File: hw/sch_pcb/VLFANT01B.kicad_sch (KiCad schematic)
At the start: 9 parts, among them J1 RJ45_RJHSE-5384, J2 RJ45_RJHSE-5384, J3 RJ45_RJHSE-5384, J7 SMA, J9 JUMP_3X2, M1 HOLE, M2 HOLE, M3 HOLE, M4 HOLE

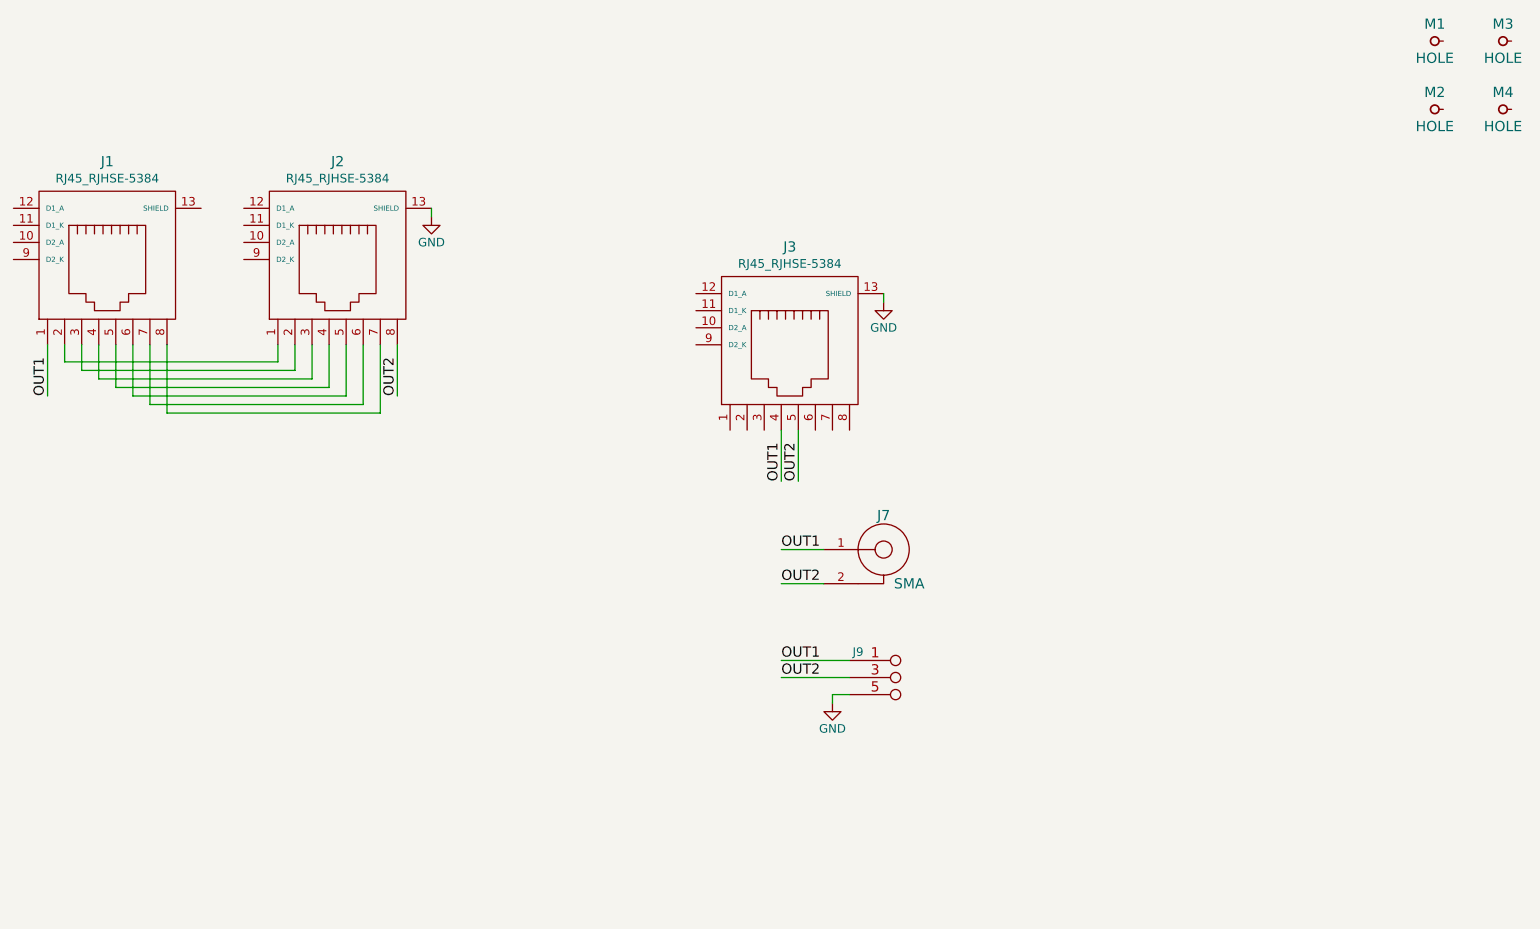
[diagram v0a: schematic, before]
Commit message: verze s narazecimi konektory
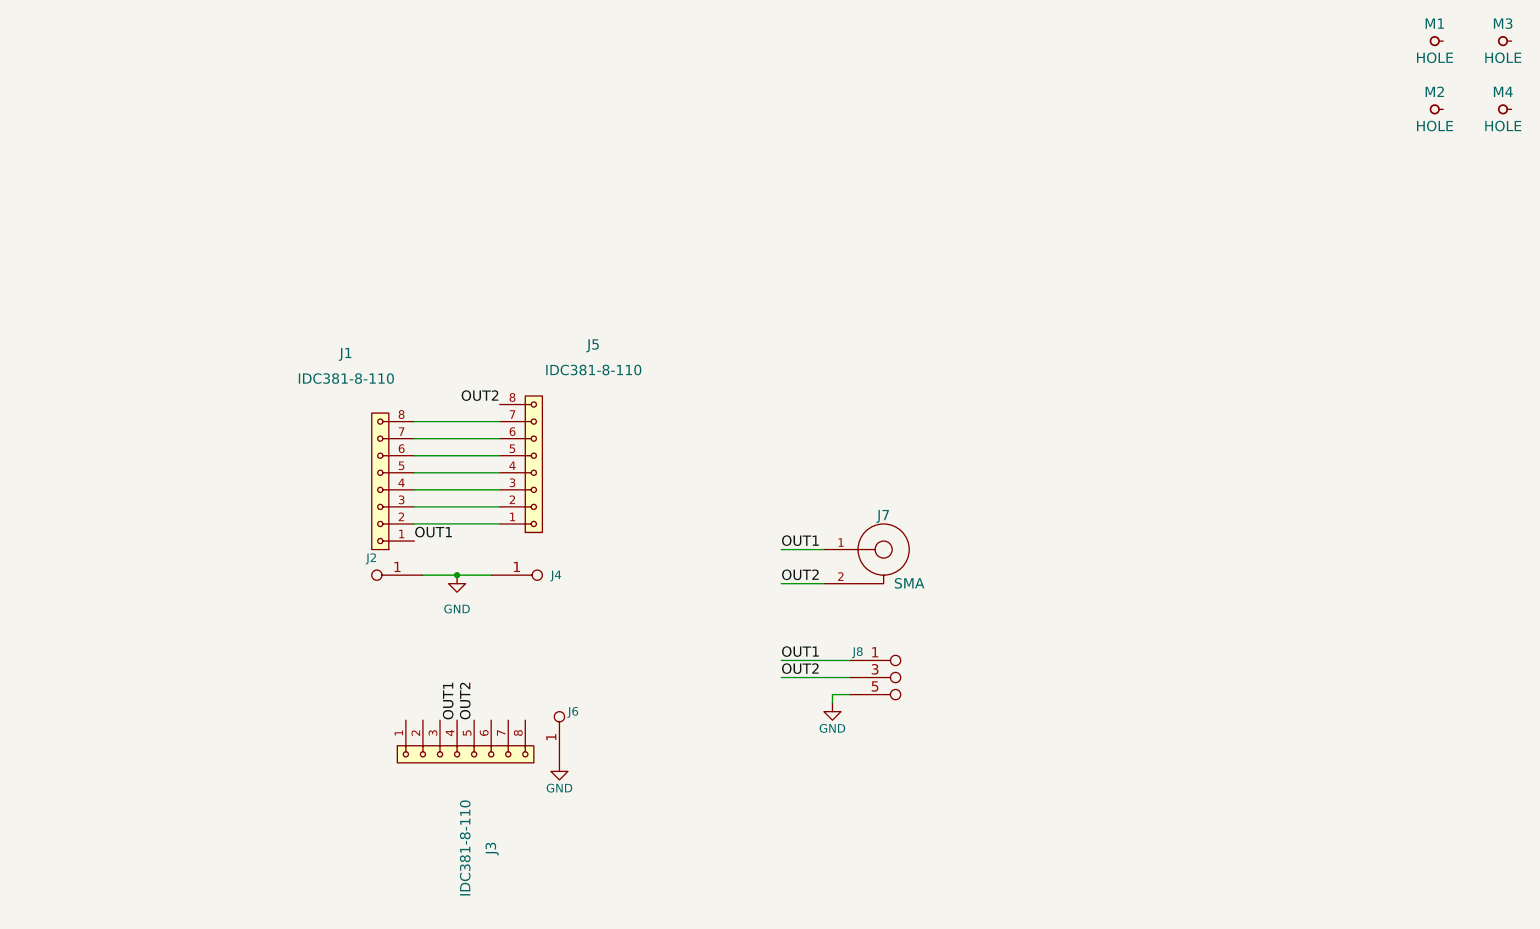
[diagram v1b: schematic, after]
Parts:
- removed J1, J2, J3: RJ45_RJHSE-5384, Mlab_CON:RJHSE-5384(RJ45), symbol VLFANT01B-rescue:RJ45_RJHSE-5384
- added J1, J3, J5: IDC381-8-110, Mlab_CON:IDC381-8-110, symbol MLAB_HEADER:HEADER_1x08
- added J2, J4, J6: JUMP_2x1, Mlab_Pin_Headers:Straight_1x01, symbol MLAB_Jumpers:JUMP_2x1
- M1, M2, M3, M4: now left out of the parts list
- renumbered J9 to J8
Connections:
- net GND: now also J2.1, J2.2 (1), J4.1, J4.2 (1), J6.1, J6.2 (1)
- net OUT1: now also J1.1, J3.4
- net OUT2: now also J3.5, J5.8
- new net: J1.2, J5.1
- new net: J1.3, J5.2
- new net: J1.4, J5.3
- new net: J1.5, J5.4
- new net: J1.6, J5.5
- new net: J1.7, J5.6
- new net: J1.8, J5.7
